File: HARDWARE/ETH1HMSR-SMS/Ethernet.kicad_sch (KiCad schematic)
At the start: 25 parts, among them J301 RJ45_Wuerth_7499010121A, U301 LAN8742A, Y301 NX5032GA-25

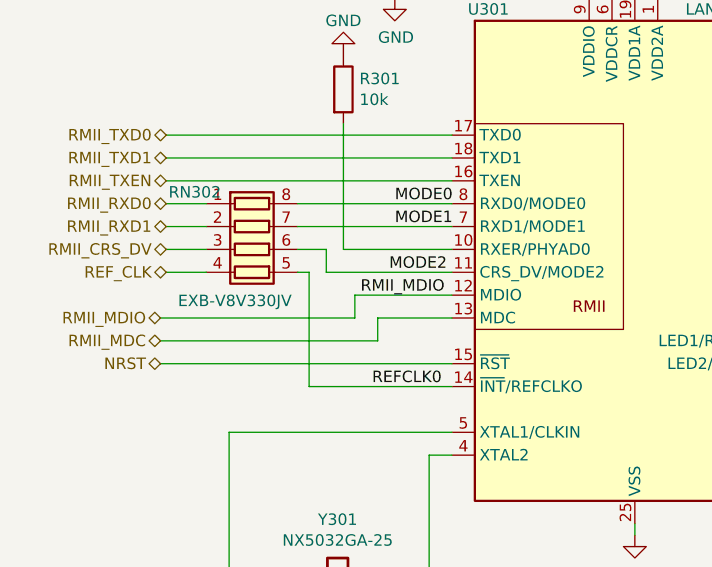
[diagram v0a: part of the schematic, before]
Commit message: PCB design
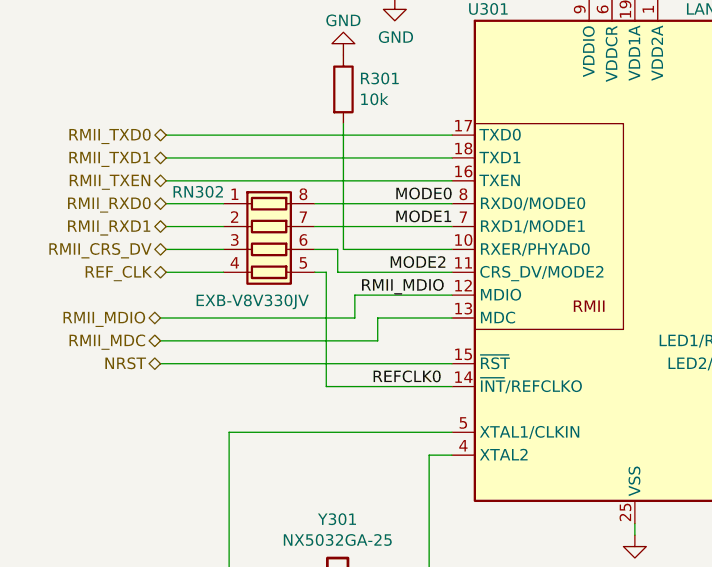
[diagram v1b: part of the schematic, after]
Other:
- moved on the sheet: RN302
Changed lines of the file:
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@@
 	(wire
 		(pts
-			(xy 65.405 83.82) (xy 60.96 83.82)
+			(xy 67.31 83.82) (xy 60.96 83.82)
 		)
 		(stroke
@@
 	(wire
 		(pts
-			(xy 60.96 86.36) (xy 65.405 86.36)
+			(xy 60.96 86.36) (xy 67.31 86.36)
 		)
 		(stroke
@@
 	(wire
 		(pts
-			(xy 60.96 91.44) (xy 65.405 91.44)
+			(xy 60.96 91.44) (xy 67.31 91.44)
 		)
 		(stroke
@@
 	(wire
 		(pts
-			(xy 75.565 86.36) (xy 92.71 86.36)
+			(xy 77.47 86.36) (xy 92.71 86.36)
 		)
 		(stroke
@@
 	(wire
 		(pts
-			(xy 60.96 88.9) (xy 65.405 88.9)
+			(xy 60.96 88.9) (xy 67.31 88.9)
 		)
 		(stroke
@@
 	(wire
 		(pts
-			(xy 76.835 104.14) (xy 92.71 104.14)
+			(xy 78.74 104.14) (xy 92.71 104.14)
 		)
 		(stroke
@@
 	(wire
 		(pts
-			(xy 76.835 91.44) (xy 76.835 104.14)
+			(xy 78.74 91.44) (xy 78.74 104.14)
 		)
 		(stroke
@@
 	(wire
 		(pts
-			(xy 75.565 83.82) (xy 92.71 83.82)
+			(xy 77.47 83.82) (xy 92.71 83.82)
 		)
 		(stroke
@@
 	(wire
 		(pts
-			(xy 75.565 91.44) (xy 76.835 91.44)
+			(xy 77.47 91.44) (xy 78.74 91.44)
 		)
 		(stroke
@@
 	(wire
 		(pts
-			(xy 78.74 91.44) (xy 92.71 91.44)
+			(xy 80.01 91.44) (xy 92.71 91.44)
 		)
 		(stroke
@@
 	(wire
 		(pts
-			(xy 75.565 88.9) (xy 78.74 88.9)
+			(xy 77.47 88.9) (xy 80.01 88.9)
 		)
 		(stroke
@@
 	(wire
 		(pts
-			(xy 78.74 88.9) (xy 78.74 91.44)
+			(xy 80.01 88.9) (xy 80.01 91.44)
 		)
 		(stroke
@@
 	(symbol
 		(lib_id "Device:R_Pack04")
-		(at 70.485 88.9 270)
+		(at 72.39 88.9 270)
 		(unit 1)
 		(exclude_from_sim no)
@@
 		(dnp no)
 		(property "Reference" "RN302"
-			(at 64.135 82.55 90)
+			(at 64.516 82.55 90)
 			(effects
 				(font
@@
 		)
 		(property "Value" "EXB-V8V330JV"
-			(at 68.58 94.615 90)
+			(at 70.485 94.615 90)
 			(effects
 				(font
@@
 		)
 		(property "Footprint" "Resistor_SMD:R_Array_Concave_4x0603"
-			(at 70.485 95.885 90)
+			(at 72.39 95.885 90)
 			(effects
 				(font
@@
 		)
 		(property "Datasheet" "~"
-			(at 70.485 88.9 0)
+			(at 72.39 88.9 0)
 			(effects
 				(font
@@
 		)
 		(property "Description" ""
-			(at 70.485 88.9 0)
-			(effects
-				(font
+			(at 72.39 88.9 0)
+			(effects
+				(font
